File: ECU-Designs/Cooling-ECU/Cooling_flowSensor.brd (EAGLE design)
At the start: 42.9 x 43.2 mm, 16 parts

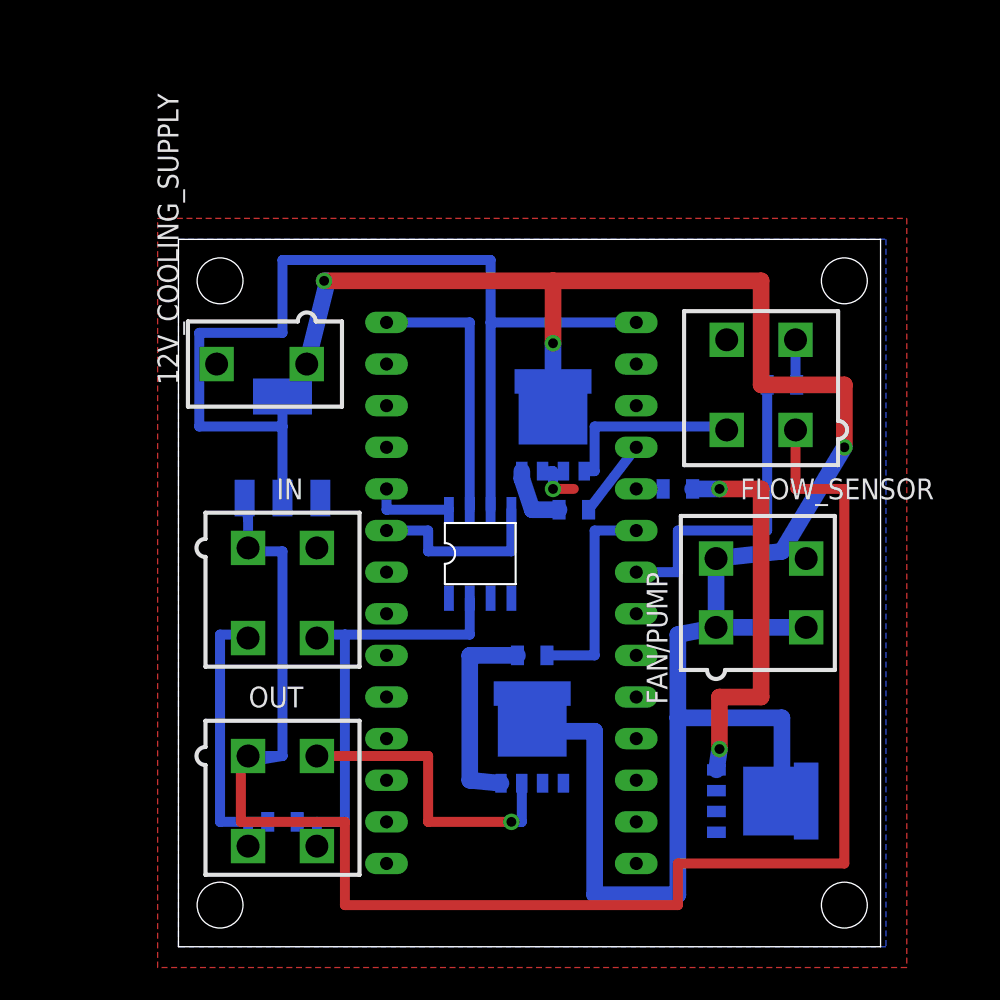
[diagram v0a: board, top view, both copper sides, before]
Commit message: Updated cooling board
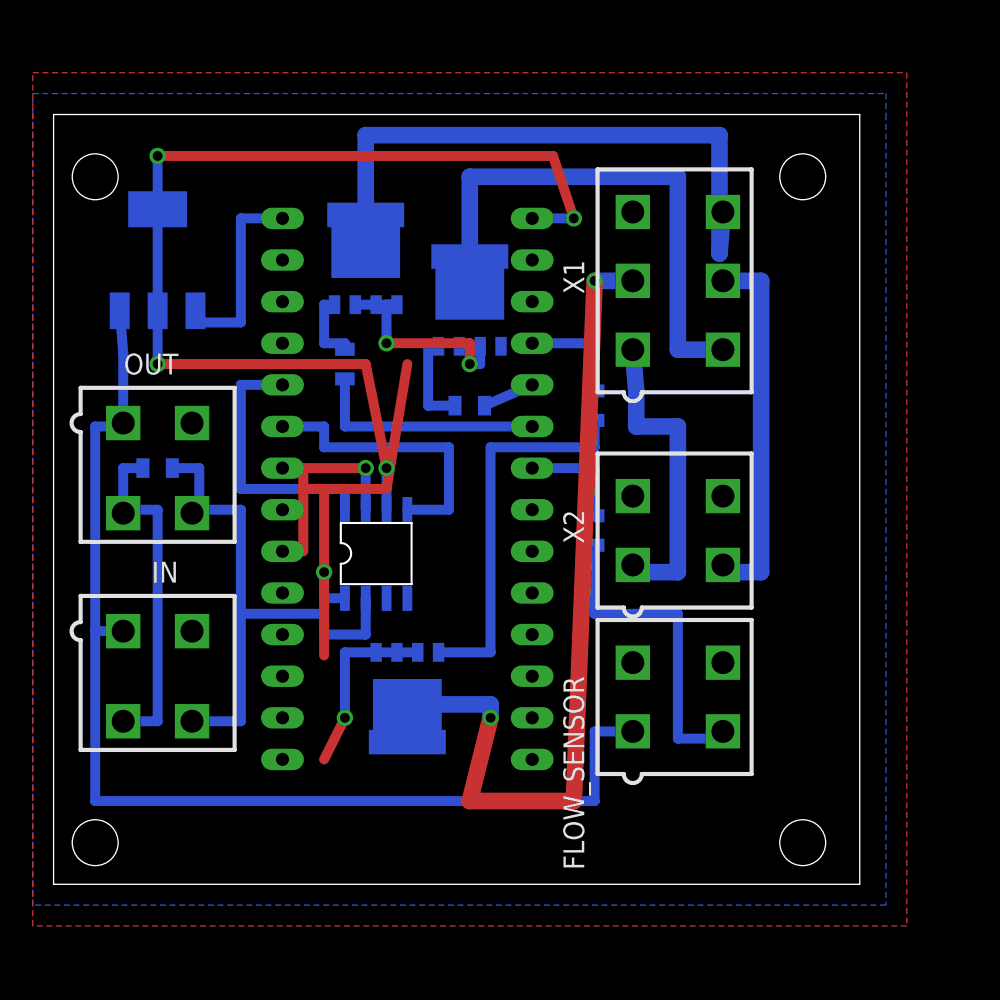
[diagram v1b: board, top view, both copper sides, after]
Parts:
- removed 12V_COOLING_SUPPLY: MINIFIT_5566-2, HyTechDevices:MINIFIT_5566-2
- removed FAN/PUMP: MINIFIT_5566-4, HyTechDevices:MINIFIT_5566-4
- added X1: MINIFIT_5566-6, HyTechDevices:MINIFIT_5566-6
- added X2: MINIFIT_5566-4, HyTechDevices:MINIFIT_5566-4
- moved U$4 35.3 mm to (38.1, 58.4), turned to 0 degrees
- moved R1 22.9 mm to (19.1, 48.3)
- moved OUT 21.7 mm to (19.1, 48.3)
- moved R4 21.1 mm to (30.5, 54.6), turned to 270 degrees
- moved FLOW_SENSOR 19.7 mm to (50.8, 34.3), turned to 270 degrees
- moved U$5 15.3 mm to (31.8, 61.0)
- moved R5 14.5 mm to (45.7, 44.5), turned to 270 degrees
- moved IC1 13.7 mm to (19.1, 61.0)
- moved R3 13.7 mm to (38.1, 52.1), turned to 180 degrees
- moved IN 9.16 mm to (19.1, 35.6)
- moved U$1 8.98 mm to (25.4, 29.2)
- moved U$3 8.03 mm to (34.3, 34.3), turned to 180 degrees
- moved R2 6.48 mm to (45.7, 52.1), turned to 270 degrees
- moved U$2 6.35 mm to (30.5, 45.7)
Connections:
- net N$11 renamed CAN-H
- net N$8 renamed CAN-L
- removed net 12V_COOLING_SUPPLY: 12V_COOLING_SUPPLY.1, FAN/PUMP.1, FAN/PUMP.2, FAN/PUMP.3, U$3.MB, U$3.MB2, U$4.MB, U$4.MB2, U$5.MB, U$5.MB2
- removed net N$4 (its old number): R2.2, U$5.4
- removed net N$6 (its old number): R4.1, U$3.4
- new net AUX_12V_1: X1.1, X2.1
- new net AUX_12V_2: X1.3
- new net AUX_12V_3: X1.5, X2.3
- new net N$13: R4.1, U$5.4
- new net N$14: U$4.MB, U$4.MB2, X1.4
- new net N$15: U$5.MB, U$5.MB2, X1.6
- new net N$19: U$3.MB, U$3.MB2, X1.2
- new net N$9: R2.2, U$3.4
- net GND: now also U$2.8
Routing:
- net 12V_COOLING_SUPPLY: track 132.6 -> 0.00 mm, vias 3 -> 0
- net N$19: track 0.00 -> 53.9 mm, vias 0 -> 2
- net N$15: track 0.00 -> 38.5 mm
- net N$14: track 0.00 -> 31.9 mm
- net 12V: track 99.6 -> 70.4 mm
- net GND: track 50.0 -> 75.8 mm, vias 2 -> 5
- net N$9: track 0.00 -> 23.7 mm
- net AUX_12V_3: track 0.00 -> 22.9 mm
- net AUX_12V_1: track 0.00 -> 19.3 mm
- net N$12: track 23.9 -> 5.90 mm, vias 2 -> 0
- net N$7: track 2.82 -> 20.1 mm
- net N$10: track 19.4 -> 6.72 mm
- net N$6 (its old number): track 12.4 -> 0.00 mm
- net N$2: track 5.08 -> 16.5 mm
- net CAN-H: track 27.6 -> 34.4 mm
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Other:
- board size 42.9 x 43.2 mm -> 49.2 x 47 mm
